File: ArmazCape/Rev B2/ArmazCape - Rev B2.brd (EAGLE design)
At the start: 85 x 70.5 mm, 167 parts, among them M1 7490100111A, Q1 32.768kHz, 12.5pF, Q2 ASE, Q4 IRLML6344TRPBF, Q5 IRLML6344TRPBF, U1 L7985A, U2 L7985A, U3 DS1307ZN+, U4 24AA256-I/SN, U5 CD4050BD, U6 CD4050BD, U7 PCA9685PW, U8 SN65HVD08D, U9 KSZ8851SNLI

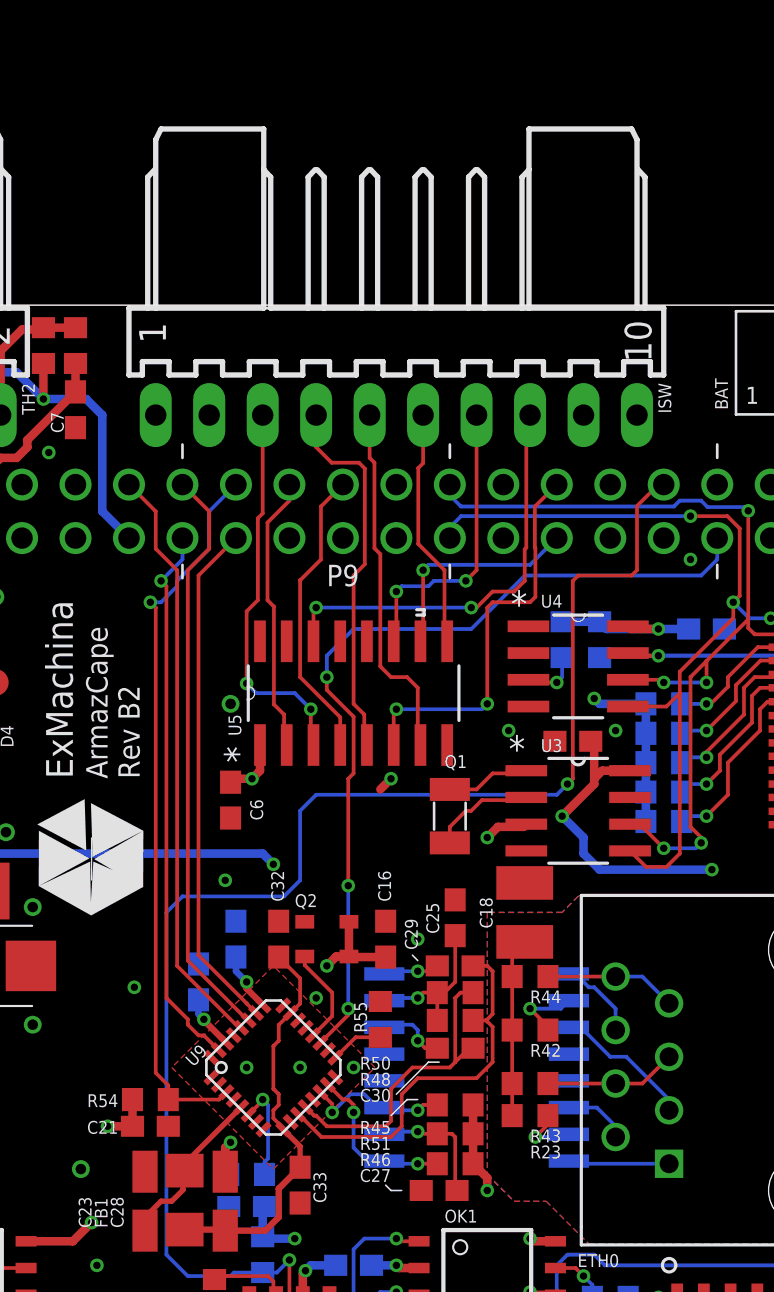
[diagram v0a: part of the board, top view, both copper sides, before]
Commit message: Added GERBER files for ArmazCape Rev B3
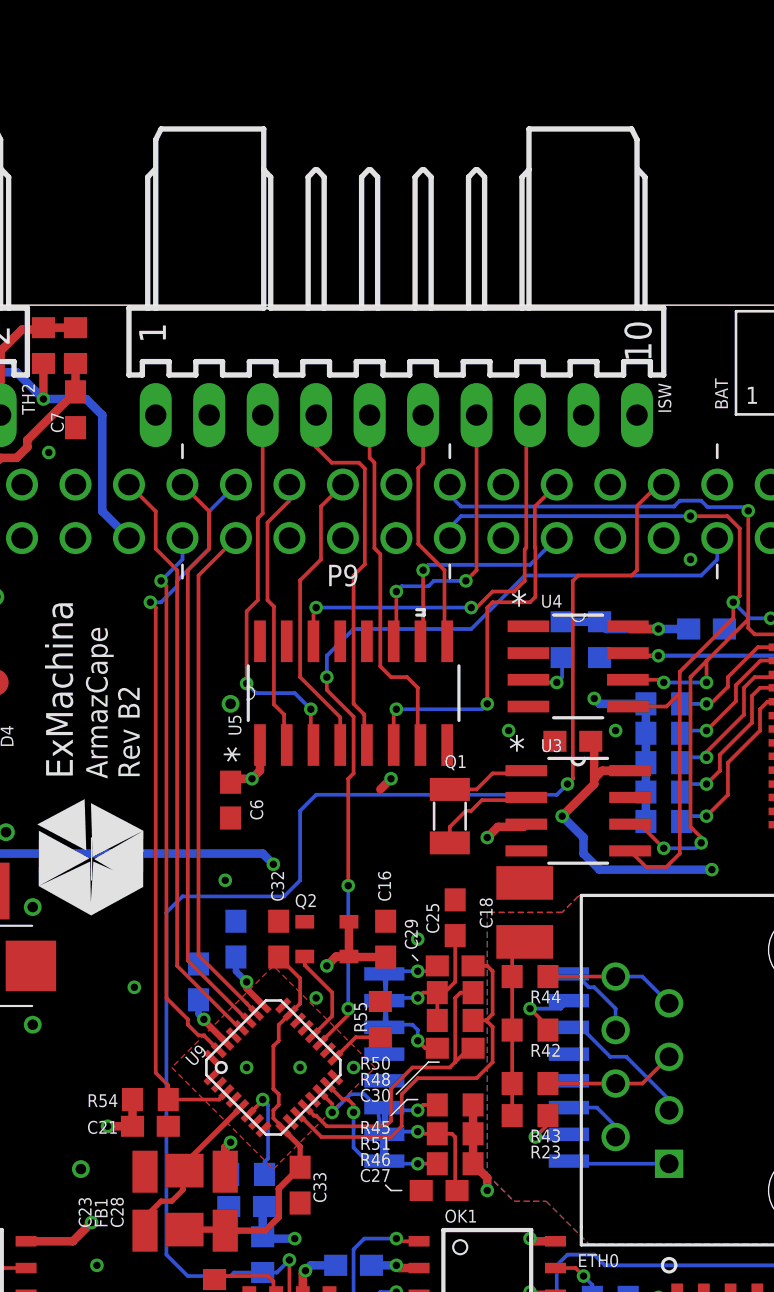
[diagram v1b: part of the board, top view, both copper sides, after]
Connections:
- net N$4: now also M1.8; no longer M1.6
- net N$4200: now also M1.1; no longer M1.3
- net N$4400: now also M1.3; no longer M1.1
- net N$51: now also M1.6; no longer M1.8
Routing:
- net N$4400: track 7.94 -> 12.7 mm
- net N$4200: track 7.01 -> 11.5 mm
- net N$51: track 2.68 -> 5.17 mm
- net N$4: track 3.33 -> 5.57 mm
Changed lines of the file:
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@@
 <setting verticaltext="up"/>
 </settings>
-<grid distance="10" unitdist="mil" unit="mil" style="lines" multiple="5" display="yes" altdistance="1" altunitdist="mil" altunit="mil"/>
+<grid distance="50" unitdist="mil" unit="mil" style="dots" multiple="2" display="yes" altdistance="25" altunitdist="mil" altunit="mil"/>
 <layers>
-<layer number="1" name="Top" color="43" fill="1" visible="yes" active="yes"/>
-<layer number="2" name="Route2" color="32" fill="1" visible="no" active="yes"/>
+<layer number="1" name="Top" color="16" fill="1" visible="yes" active="yes"/>
+<layer number="2" name="Route2" color="17" fill="1" visible="no" active="yes"/>
 <layer number="3" name="Route3" color="4" fill="3" visible="no" active="no"/>
 <layer number="14" name="Route14" color="1" fill="6" visible="no" active="no"/>
-<layer number="15" name="Route15" color="38" fill="1" visible="no" active="yes"/>
-<layer number="16" name="Bottom" color="17" fill="1" visible="no" active="yes"/>
-<layer number="17" name="Pads" color="2" fill="1" visible="yes" active="yes"/>
-<layer number="18" name="Vias" color="2" fill="1" visible="yes" active="yes"/>
+<layer number="15" name="Route15" color="19" fill="1" visible="no" active="yes"/>
+<layer number="16" name="Bottom" color="21" fill="1" visible="yes" active="yes"/>
+<layer number="17" name="Pads" color="18" fill="1" visible="yes" active="yes"/>
+<layer number="18" name="Vias" color="38" fill="1" visible="yes" active="yes"/>
 <layer number="19" name="Unrouted" color="6" fill="1" visible="yes" active="yes"/>
-<layer number="20" name="Dimension" color="26" fill="1" visible="yes" active="yes"/>
-<layer number="21" name="tPlace" color="7" fill="1" visible="yes" active="yes"/>
-<layer number="22" name="bPlace" color="7" fill="1" visible="no" active="yes"/>
-<layer number="23" name="tOrigins" color="15" fill="1" visible="yes" active="yes"/>
-<layer number="24" name="bOrigins" color="15" fill="1" visible="no" active="yes"/>
-<layer number="25" name="tNames" color="7" fill="1" visible="yes" active="yes"/>
-<layer number="26" name="bNames" color="7" fill="1" visible="no" active="yes"/>
-<layer number="27" name="tValues" color="7" fill="1" visible="yes" active="yes"/>
-<layer number="28" name="bValues" color="7" fill="1" visible="no" active="yes"/>
+<layer number="20" name="Dimension" color="7" fill="1" visible="yes" active="yes"/>
+<layer number="21" name="tPlace" color="55" fill="1" visible="no" active="yes"/>
+<layer number="22" name="bPlace" color="54" fill="1" visible="yes" active="yes"/>
+<layer number="23" name="tOrigins" color="15" fill="1" visible="no" active="yes"/>
+<layer number="24" name="bOrigins" color="15" fill="1" visible="yes" active="yes"/>
+<layer number="25" name="tNames" color="55" fill="1" visible="no" active="yes"/>
+<layer number="26" name="bNames" color="54" fill="1" visible="yes" active="yes"/>
+<layer number="27" name="tValues" color="53" fill="1" visible="no" active="yes"/>
+<layer number="28" name="bValues" color="52" fill="1" visible="yes" active="yes"/>
 <layer number="29" name="tStop" color="7" fill="3" visible="no" active="yes"/>
 <layer number="30" name="bStop" color="7" fill="6" visible="no" active="yes"/>
@@
 <layer number="38" name="bTest" color="7" fill="1" visible="no" active="yes"/>
 <layer number="39" name="tKeepout" color="4" fill="11" visible="no" active="yes"/>
-<layer number="40" name="bKeepout" color="1" fill="11" visible="no" active="yes"/>
+<layer number="40" name="bKeepout" color="3" fill="11" visible="no" active="yes"/>
 <layer number="41" name="tRestrict" color="4" fill="10" visible="no" active="yes"/>
-<layer number="42" name="bRestrict" color="1" fill="10" visible="no" active="yes"/>
+<layer number="42" name="bRestrict" color="3" fill="10" visible="no" active="yes"/>
 <layer number="43" name="vRestrict" color="2" fill="10" visible="no" active="yes"/>
-<layer number="44" name="Drills" color="7" fill="1" visible="no" active="yes"/>
-<layer number="45" name="Holes" color="7" fill="1" visible="no" active="yes"/>
-<layer number="46" name="Milling" color="3" fill="1" visible="no" active="yes"/>
-<layer number="47" name="Measures" color="7" fill="1" visible="yes" active="yes"/>
-<layer number="48" name="Document" color="7" fill="1" visible="no" active="yes"/>
-<layer number="49" name="Reference" color="7" fill="1" visible="no" active="yes"/>
+<layer number="44" name="Drills" color="16" fill="1" visible="no" active="yes"/>
+<layer number="45" name="Holes" color="35" fill="1" visible="no" active="yes"/>
+<layer number="46" name="Milling" color="35" fill="1" visible="no" active="yes"/>
+<layer number="47" name="Measures" color="21" fill="1" visible="yes" active="yes"/>
+<layer number="48" name="Document" color="24" fill="1" visible="no" active="yes"/>
+<layer number="49" name="Reference" color="48" fill="1" visible="no" active="yes"/>
 <layer number="50" name="dxf" color="7" fill="1" visible="no" active="no"/>
-<layer number="51" name="tDocu" color="7" fill="1" visible="no" active="yes"/>
-<layer number="52" name="bDocu" color="7" fill="1" visible="no" active="yes"/>
+<layer number="51" name="tDocu" color="55" fill="1" visible="no" active="yes"/>
+<layer number="52" name="bDocu" color="54" fill="1" visible="yes" active="yes"/>
 <layer number="53" name="tGND_GNDA" color="7" fill="1" visible="no" active="no"/>
 <layer number="54" name="bGND_GNDA" color="7" fill="1" visible="no" active="no"/>
@@
 <layer number="100" name="Mechanical" color="7" fill="1" visible="yes" active="yes"/>
 <layer number="101" name="Patch_Top" color="7" fill="1" visible="no" active="yes"/>
-<layer number="102" name="Vscore" color="7" fill="1" visible="no" active="yes"/>
+<layer number="102" name="Vscore" color="13" fill="1" visible="no" active="yes"/>
 <layer number="103" name="Top_middle" color="7" fill="1" visible="no" active="yes"/>
 <layer number="104" name="Name" color="7" fill="1" visible="no" active="yes"/>
@@
 <wire x1="47.244" y1="32.1564" x2="47.244" y2="32.55665625" width="0.1778" layer="1"/>
 <wire x1="47.244" y1="32.55665625" x2="46.68445625" y2="33.1162" width="0.1778" layer="1"/>
-<contactref element="M1" pad="3"/>
+<contactref element="M1" pad="1"/>
 <wire x1="52.236" y1="32.512" x2="51.562" y2="32.512" width="0.1778" layer="1"/>
 <wire x1="51.562" y1="32.512" x2="51.308" y2="32.258" width="0.1778" layer="1"/>
 <via x="51.308" y="32.258" extent="1-16" drill="0.35"/>
 <wire x1="51.308" y1="32.258" x2="49.844" y2="32.258" width="0.1778" layer="16"/>
-<wire x1="49.844" y1="32.258" x2="49.717" y2="32.385" width="0.1778" layer="16"/>
-<wire x1="49.717" y1="32.385" x2="49.403" y2="32.385" width="0.1778" layer="16"/>
+<wire x1="49.844" y1="32.258" x2="49.717" y2="29.845" width="0.1778" layer="16"/>
+<wire x1="49.717" y1="29.845" x2="49.403" y2="32.385" width="0.1778" layer="16"/>
 <wire x1="49.403" y1="32.385" x2="48.768" y2="33.02" width="0.1778" layer="16"/>
 <wire x1="48.768" y1="33.02" x2="48.1076" y2="33.02" width="0.1778" layer="16"/>
@@
 <signal name="N$51">
 <contactref element="C29" pad="2"/>
-<contactref element="M1" pad="8"/>
+<contactref element="M1" pad="6"/>
 <via x="51.308" y="38.862" extent="1-16" drill="0.35"/>
 <wire x1="51.308" y1="38.862" x2="49.844" y2="38.862" width="0.1778" layer="16"/>
-<wire x1="49.844" y1="38.862" x2="49.717" y2="38.735" width="0.1778" layer="16"/>
+<wire x1="49.844" y1="38.862" x2="49.717" y2="36.195" width="0.1778" layer="16"/>
 <wire x1="51.308" y1="38.862" x2="51.982" y2="38.862" width="0.1778" layer="1"/>
 <wire x1="51.982" y1="38.862" x2="52.236" y2="39.116" width="0.1778" layer="1"/>
@@
 <contactref element="R46" pad="1"/>
 <contactref element="U9" pad="15"/>
-<contactref element="M1" pad="1"/>
+<contactref element="M1" pad="3"/>
 <wire x1="47.038009375" y1="33.469753125" x2="47.7417625" y2="32.766" width="0.1778" layer="1"/>
 <wire x1="47.7417625" y1="32.766" x2="48.006" y2="32.766" width="0.1778" layer="1"/>
@@
 <wire x1="48.26" y1="30.48" x2="48.768" y2="29.972" width="0.1778" layer="16"/>
 <wire x1="48.768" y1="29.972" x2="49.59" y2="29.972" width="0.1778" layer="16"/>
-<wire x1="49.59" y1="29.972" x2="49.717" y2="29.845" width="0.1778" layer="16"/>
+<wire x1="49.59" y1="29.972" x2="49.717" y2="32.385" width="0.1778" layer="16"/>
 <wire x1="52.236" y1="29.718" x2="51.308" y2="29.718" width="0.1778" layer="1"/>
 <via x="51.308" y="29.718" extent="1-16" drill="0.35"/>
 <wire x1="51.308" y1="29.718" x2="49.844" y2="29.718" width="0.1778" layer="16"/>
-<wire x1="49.844" y1="29.718" x2="49.717" y2="29.845" width="0.1778" layer="16"/>
+<wire x1="49.844" y1="29.718" x2="49.717" y2="32.385" width="0.1778" layer="16"/>
 <wire x1="48.006" y1="32.766" x2="48.26" y2="32.512" width="0.1778" layer="1"/>
 <wire x1="48.26" y1="32.512" x2="48.26" y2="32.1564" width="0.1778" layer="1"/>
 </signal>
 <signal name="N$4">
-<contactref element="M1" pad="6"/>
+<contactref element="M1" pad="8"/>
 <contactref element="C30" pad="2"/>
 <wire x1="52.236" y1="35.2044" x2="51.6636" y2="35.2044" width="0.1778" layer="1"/>
@@
 <wire x1="51.308" y1="36.068" x2="51.054" y2="36.322" width="0.1778" layer="16"/>
 <wire x1="51.054" y1="36.322" x2="49.844" y2="36.322" width="0.1778" layer="16"/>
-<wire x1="49.844" y1="36.322" x2="49.717" y2="36.195" width="0.1778" layer="16"/>
+<wire x1="49.844" y1="36.322" x2="49.717" y2="38.735" width="0.1778" layer="16"/>
 </signal>
 <signal name="N$52">
